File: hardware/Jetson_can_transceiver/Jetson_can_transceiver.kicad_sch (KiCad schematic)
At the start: 5 parts, among them U1 MCP2551-I-P, U2 MCP2551-I-P

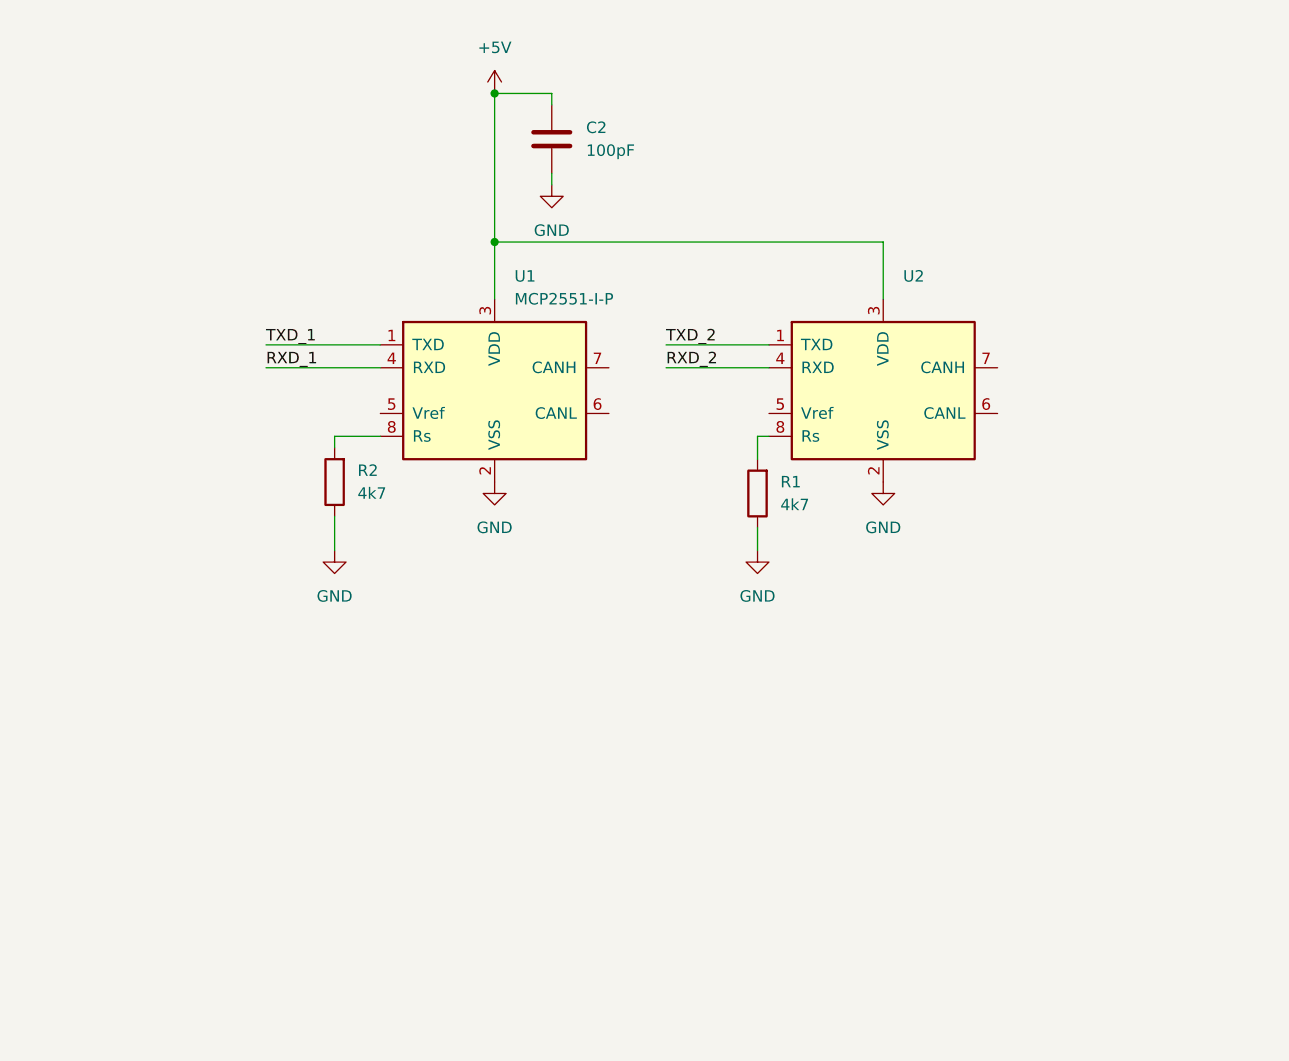
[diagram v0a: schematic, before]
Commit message: Completed blueprint for 2 transceivers
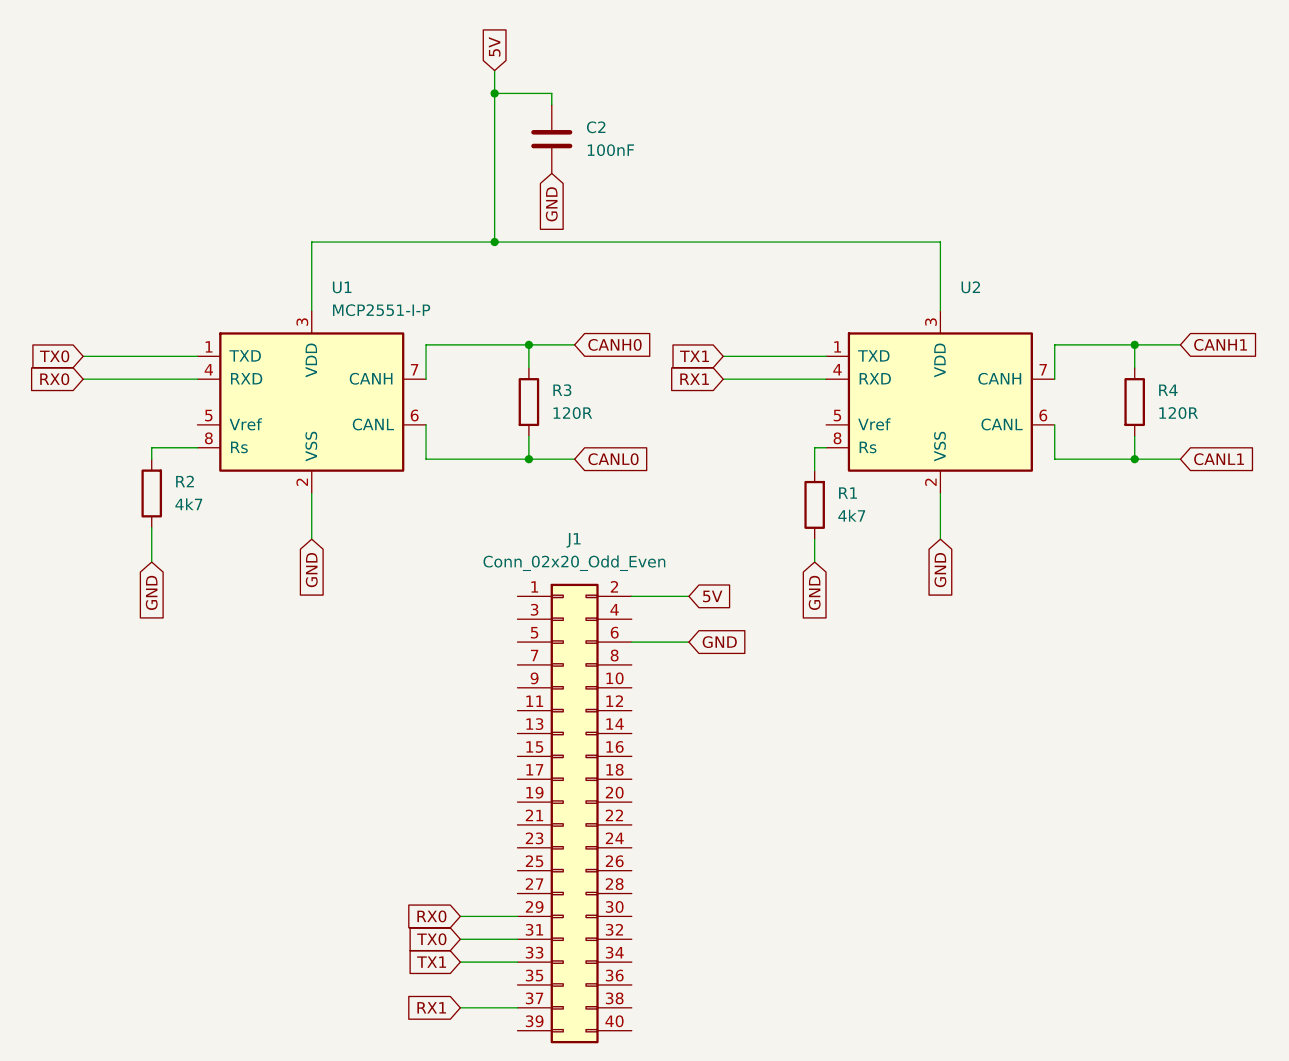
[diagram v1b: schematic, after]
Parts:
- added J1: Conn_02x20_Odd_Even, symbol Connector_Generic:Conn_02x20_Odd_Even
- added R3, R4: 120R, Resistor_SMD:R_0805_2012Metric, symbol Device:R
- C2: value 100pF -> 100nF
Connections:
- net GND: now also J1.6 (Pin_6)
- net CANL1: now reaches U2.6 (CANL)
- net CANL1: now also R4.2
- net CANH1: now reaches U2.7 (CANH)
- net CANH1: now also R4.1
- net CANL0: now reaches U1.6 (CANL)
- net CANL0: now also R3.2
- net CANH0: now reaches U1.7 (CANH)
- net CANH0: now also R3.1
- net +5V renamed 5V
- net 5V: now also J1.2 (Pin_2)
- net RXD_1 renamed RX0
- net RX0: now also J1.29 (Pin_29)
- net RXD_2 renamed RX1
- net RX1: now also J1.37 (Pin_37)
- net TXD_1 renamed TX0
- net TX0: now also J1.31 (Pin_31)
- net TXD_2 renamed TX1
- net TX1: now also J1.33 (Pin_33)
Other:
- moved on the sheet: R1, R2, U1, U2
